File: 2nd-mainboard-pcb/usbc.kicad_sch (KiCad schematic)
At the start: 13 parts, among them J1 USB_C_Receptacle, U2 PTS647SM38SMTR2LFS, U5 FT232RL

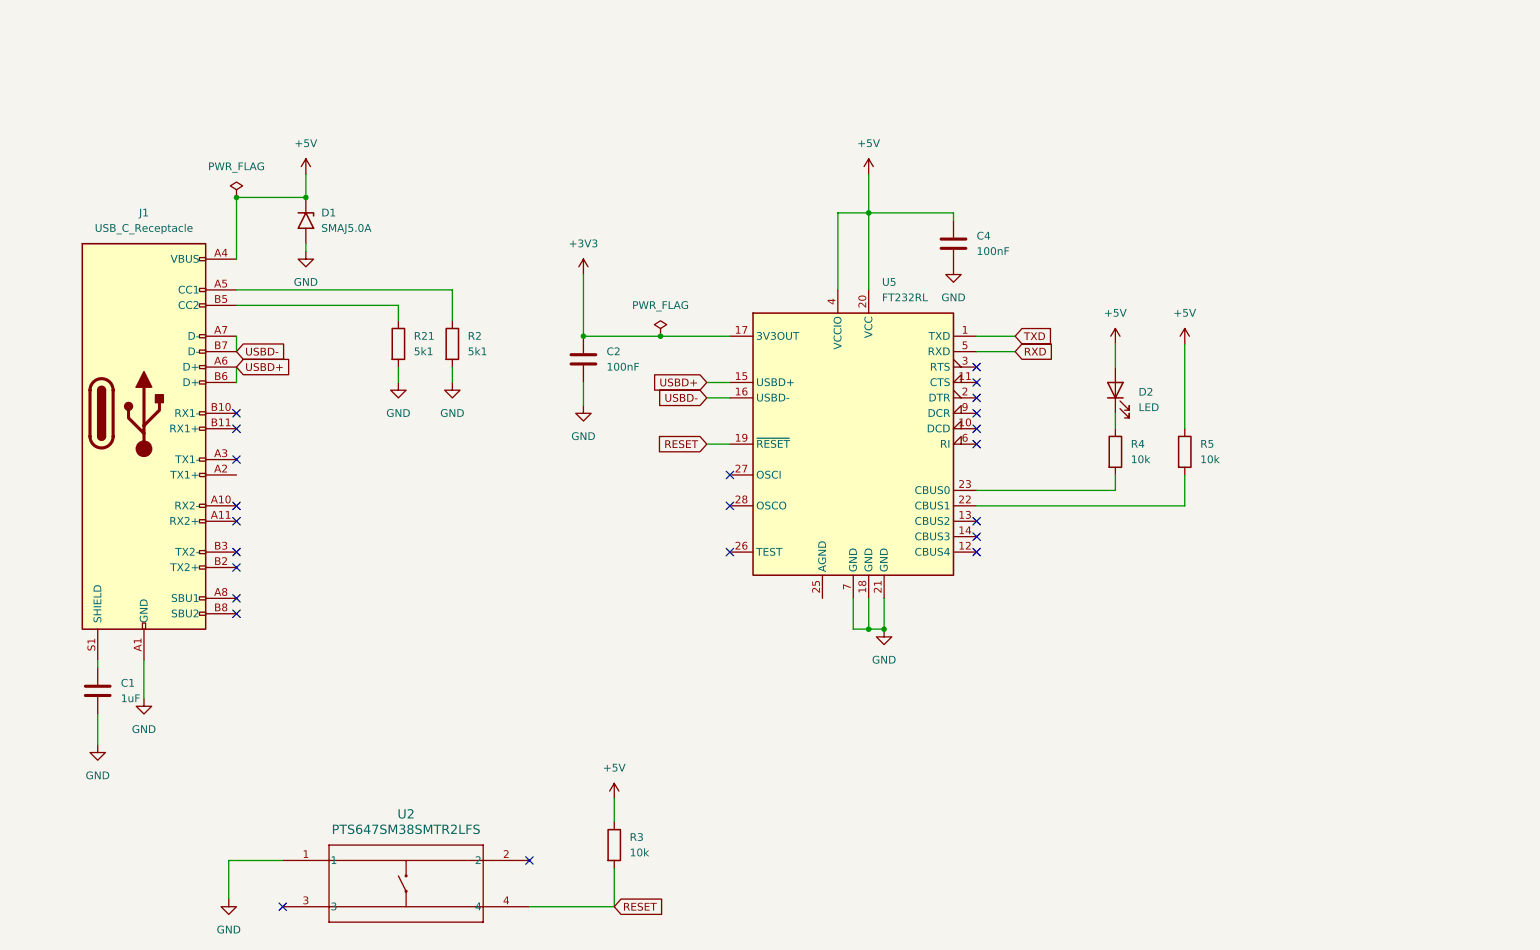
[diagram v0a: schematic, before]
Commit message: finished stacked design, annotaded
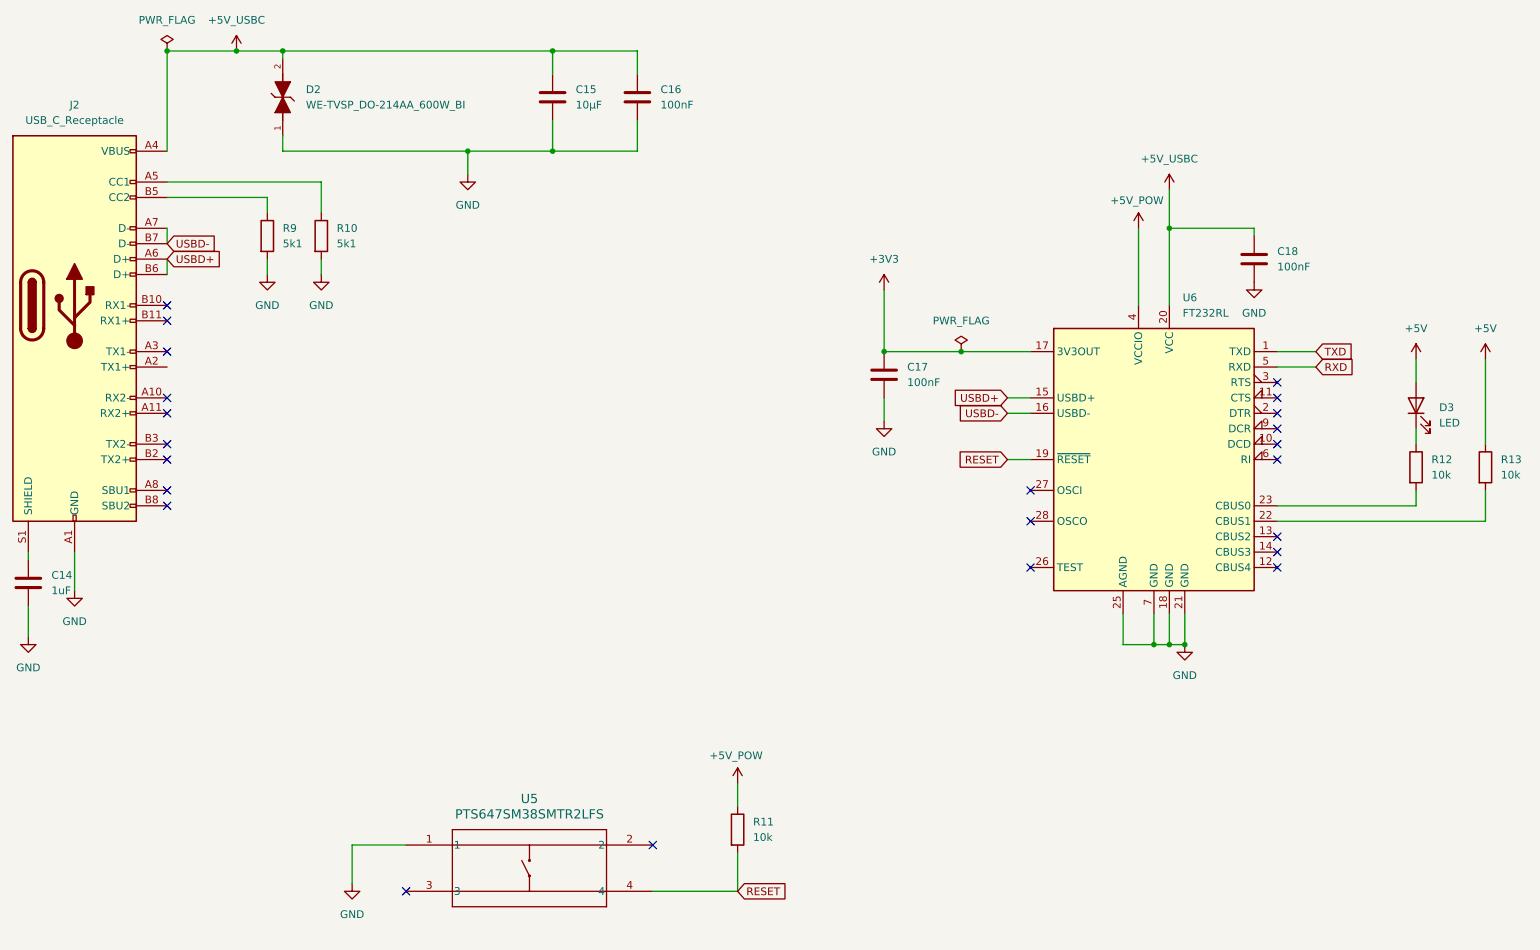
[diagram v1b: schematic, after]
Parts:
- removed D1: SMAJ5.0A, Diode_SMD:D_SMA, symbol Diode:SMAJ5.0A
- added C15: 10µF, symbol Device:C
- added C16: 100nF, symbol Device:C
- added D2: WE-TVSP_DO-214AA_600W_BI, WE-TVSP_DO-214AA_600W_BI:WE-TVSP_DO-214AA_BIDIRECTIONAL, symbol Imported_Component_Symbols:WE-TVSP_DO-214AA_600W_BI
- U5: renamed from U2; footprint SW_PTS647SM38SMTR2LFS_CNK -> Imported_Component_Footprints:SW_PTS647SM38SMTR2LFS_CNK
- renumbered C1 to C14, C2 to C17, C4 to C18, D2 to D3, J1 to J2, R2 to R10, R3 to R11, R4 to R12, R5 to R13, R21 to R9, U5 to U6
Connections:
- net +5V: no longer C18.1, J2.A4 (VBUS), J2.A9 (VBUS), J2.B4 (VBUS), J2.B9 (VBUS), R11.1, U6.20 (VCC), U6.4 (VCCIO)
- net GND: now also U6.25 (AGND), C15.2, C16.2, D2.1
- new net +5V_POW: R11.1, U6.4 (VCCIO)
- new net +5V_USBC: C15.1, C16.1, C18.1, D2.2, J2.A4 (VBUS), J2.A9 (VBUS), J2.B4 (VBUS), J2.B9 (VBUS), U6.20 (VCC)
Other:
- moved on the sheet: C14, C17, C18, D3, J2, R10, R11, R12, R13, R9, U5, U6
